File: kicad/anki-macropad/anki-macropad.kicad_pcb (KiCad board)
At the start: 2 copper layers, 99.2 x 62.1 mm, 48 parts, among them J1 USB_C_Receptacle_USB2.0_14P, SW1 PTS810 SJK 250 SMTR LFS, U1 NCP1117-3.3_SOT223, U2 W25Q128JVS, U3 RP2040, U4 USBLC6-2SC6, X1 ABM8-272-T3

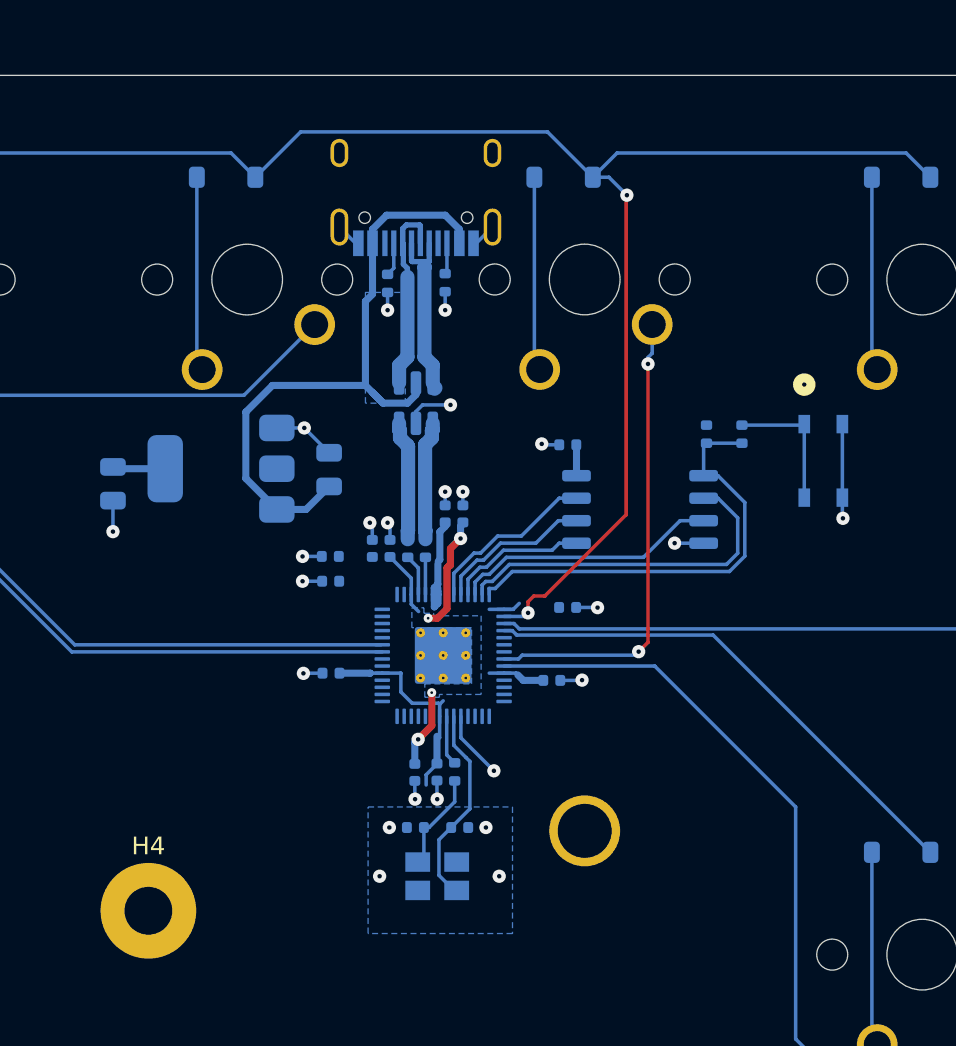
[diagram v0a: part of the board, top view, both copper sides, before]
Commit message: Finished PCB design including DRC
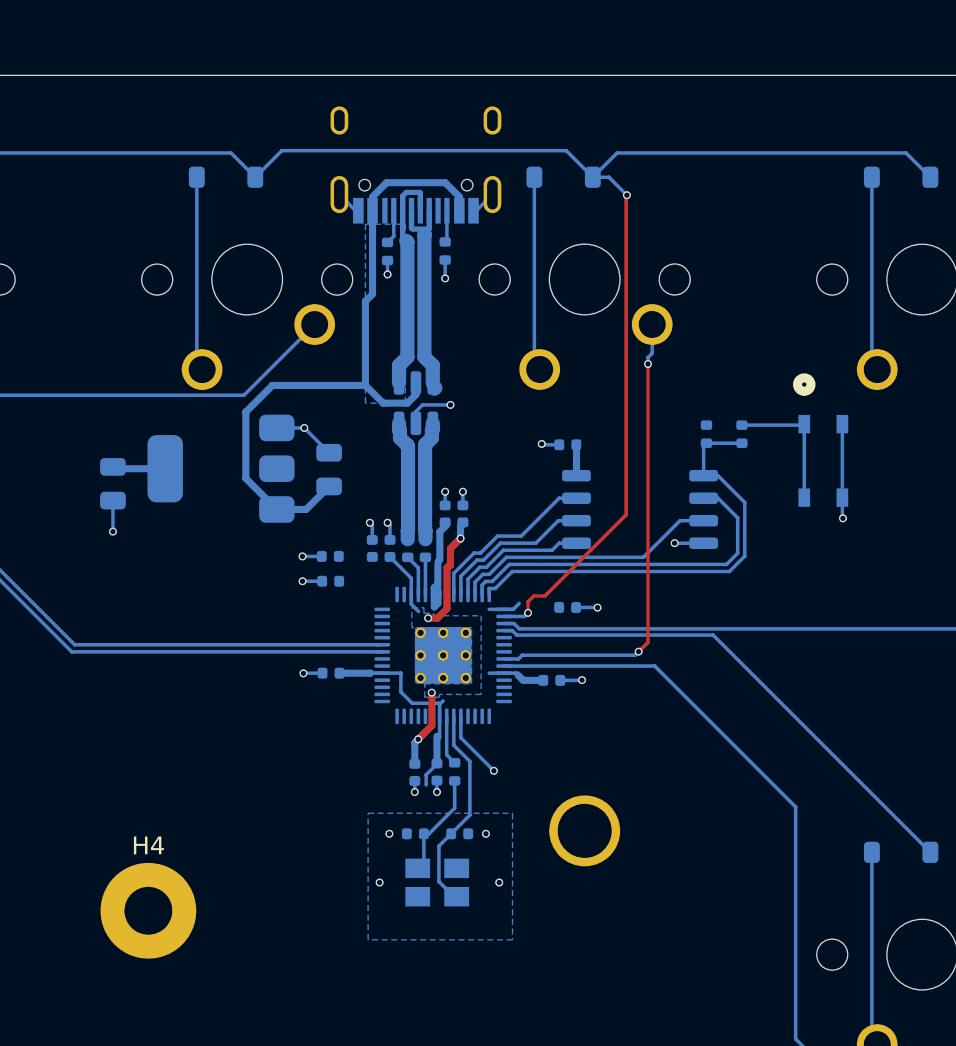
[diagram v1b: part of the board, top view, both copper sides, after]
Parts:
- moved J1 1.84 mm to (85.4, 37.1)
- moved R6 1.80 mm to (83.8, 43.4)
- moved R7 1.79 mm to (87.1, 43.4)
- moved C2 0.36 mm to (87.9, 76.3)
- moved C3 0.36 mm to (85.4, 76.3)
- moved X1 0.36 mm to (86.6, 79.0)
- turned R3 to -90 degrees
- turned R4 to -90 degrees
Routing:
- net /USB_D-: track 11.1 -> 13.0 mm
- net /USB_D+: track 9.88 -> 11.6 mm
- net GND: track 36.2 -> 34.9 mm
- net /ROW 0: track 91.6 -> 90.7 mm
